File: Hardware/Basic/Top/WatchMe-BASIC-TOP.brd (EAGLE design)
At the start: 38 x 38 mm, 62 parts, among them SW1 SWITCH.MOM, SW2 SWITCH.MOM, U2 NRF52832_MODULE_MDBT42, U4 PCF8523, U5 FT231XS

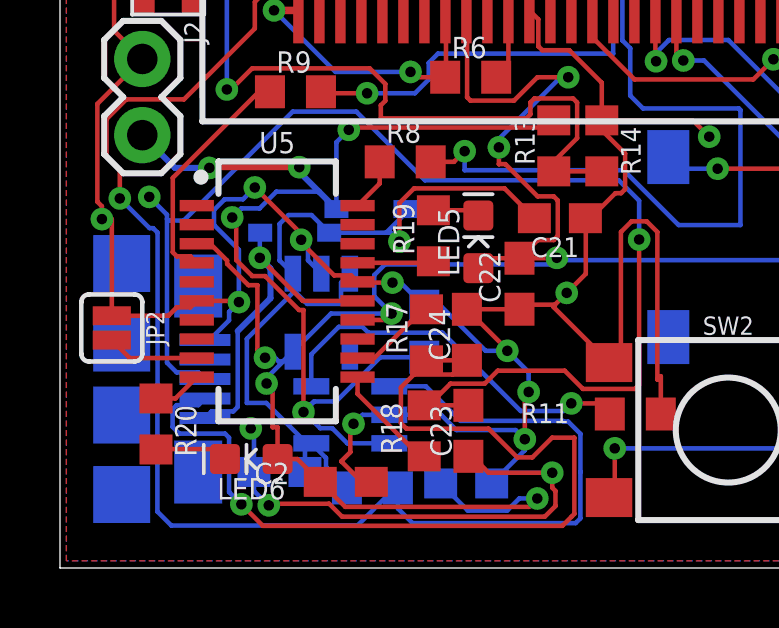
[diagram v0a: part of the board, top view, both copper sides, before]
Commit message: fixed remaining warnings
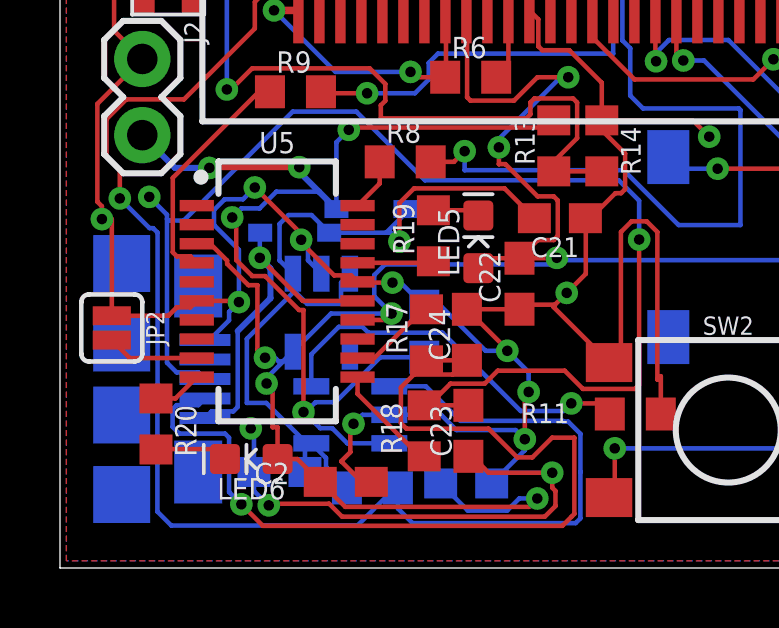
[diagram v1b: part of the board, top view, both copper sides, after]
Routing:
- net VLIPO: track 37.6 -> 36.5 mm
- net GND: track 296.9 -> 296.1 mm
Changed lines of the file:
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@@
 <wire x1="14.247" y1="18.5866" x2="14.2386" y2="18.595" width="0.1524" layer="1"/>
 <wire x1="14.2386" y1="19.4764875" x2="14.2386" y2="18.595" width="0.1524" layer="1"/>
-<wire x1="8.7122" y1="9.8091" x2="8.7122" y2="10.30668125" width="0.1524" layer="16"/>
 <wire x1="14.8844" y1="19.9152" x2="14.9352" y2="19.966" width="0.1524" layer="1"/>
 <wire x1="14.9352" y1="19.966" x2="14.9352" y2="20.7518" width="0.1524" layer="1"/>
@@
 <wire x1="12.7047" y1="5.1054" x2="10.9775" y2="5.1054" width="0.1524" layer="16"/>
 <wire x1="15.1892" y1="4.5974" x2="13.2127" y2="4.5974" width="0.1524" layer="16"/>
-<wire x1="10.9775" y1="5.1054" x2="10.7743" y2="4.9022" width="0.1524" layer="16"/>
 <wire x1="9.6774" y1="4.699" x2="9.78376875" y2="4.80536875" width="0.1524" layer="1"/>
 <via x="9.78376875" y="4.80536875" extent="1-16" drill="0.35"/>
@@
 <contactref element="C20" pad="1"/>
 <contactref element="R13" pad="2"/>
-<wire x1="12.1412" y1="7.024" x2="11.9966" y2="7.1686" width="0.2032" layer="16"/>
 <wire x1="9.2132" y1="11.9634" x2="9.2132" y2="14.1916" width="0.1524" layer="16"/>
 <wire x1="9.2132" y1="14.1916" x2="9.6266" y2="14.605" width="0.1524" layer="16"/>
@@
 <wire x1="9.6266" y1="14.605" x2="9.7028" y2="14.6812" width="0.1524" layer="1"/>
 <wire x1="16.2188" y1="14.6812" x2="16.4592" y2="14.9216" width="0.1524" layer="1"/>
-<via x="5.7404" y="11.684" extent="1-16" drill="0.35"/>
 <wire x1="5.8751" y1="11.5493" x2="5.7404" y2="11.684" width="0.1524" layer="1"/>
 <wire x1="5.8751" y1="10.26425" x2="5.8751" y2="11.5493" width="0.1524" layer="1"/>
-<wire x1="5.7404" y1="11.684" x2="6.0198" y2="11.9634" width="0.1524" layer="16"/>
 <wire x1="9.2132" y1="11.9634" x2="8.6325" y2="12.5441" width="0.2032" layer="16"/>
 <wire x1="8.6325" y1="12.5441" x2="7.9756" y2="13.201" width="0.2032" layer="16"/>
@@
 <via x="8.11565" y="5.199" extent="1-16" drill="0.35"/>
 <wire x1="8.11565" y1="5.199" x2="8.11565" y2="8.5979" width="0.1524" layer="1"/>
-<wire x1="8.125825" y1="5.209175" x2="8.43425" y2="5.5176" width="0.1524" layer="16"/>
 <wire x1="8.125825" y1="5.209175" x2="8.11565" y2="5.199" width="0.1524" layer="16"/>
 <wire x1="9.0719875" y1="4.659" x2="8.676" y2="4.659" width="0.1524" layer="16"/>
@@
 <wire x1="10.9775" y1="4.1554" x2="9.5755875" y2="4.1554" width="0.1524" layer="16"/>
 <wire x1="9.5755875" y1="4.1554" x2="9.0719875" y2="4.659" width="0.1524" layer="16"/>
-<wire x1="8.11565" y1="5.199" x2="8.46845" y2="5.5518" width="0.1524" layer="16"/>
-<wire x1="8.46845" y1="5.5518" x2="9.2033875" y2="5.5518" width="0.1524" layer="16"/>
-<wire x1="9.2033875" y1="5.5518" x2="10.6755875" y2="7.024" width="0.1524" layer="16"/>
+<wire x1="8.11565" y1="5.199" x2="8.19185" y2="5.199" width="0.1524" layer="16"/>
+<wire x1="8.51925" y1="5.5264" x2="8.19185" y2="5.199" width="0.1524" layer="16"/>
+<wire x1="8.51925" y1="5.5264" x2="9.1779875" y2="5.5264" width="0.1524" layer="16"/>
+<wire x1="9.1779875" y1="5.5264" x2="10.6755875" y2="7.024" width="0.1524" layer="16"/>
 <wire x1="10.6755875" y1="7.024" x2="12.1412" y2="7.024" width="0.1524" layer="16"/>
-<wire x1="5.7404" y1="11.684" x2="6.0424" y2="11.986" width="0.1524" layer="16"/>
 <wire x1="7.21218125" y1="12.5441" x2="8.6325" y2="12.5441" width="0.1524" layer="16"/>
 <wire x1="6.0424" y1="11.986" x2="6.65408125" y2="11.986" width="0.1524" layer="16"/>
 <wire x1="6.65408125" y1="11.986" x2="7.21218125" y2="12.5441" width="0.1524" layer="16"/>
+<via x="5.7404" y="11.684" extent="1-16" drill="0.35"/>
+<wire x1="5.7404" y1="11.684" x2="6.0424" y2="11.986" width="0.1524" layer="16"/>
 </signal>
 <signal name="V_USB">
